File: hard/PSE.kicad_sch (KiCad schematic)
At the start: 0 parts

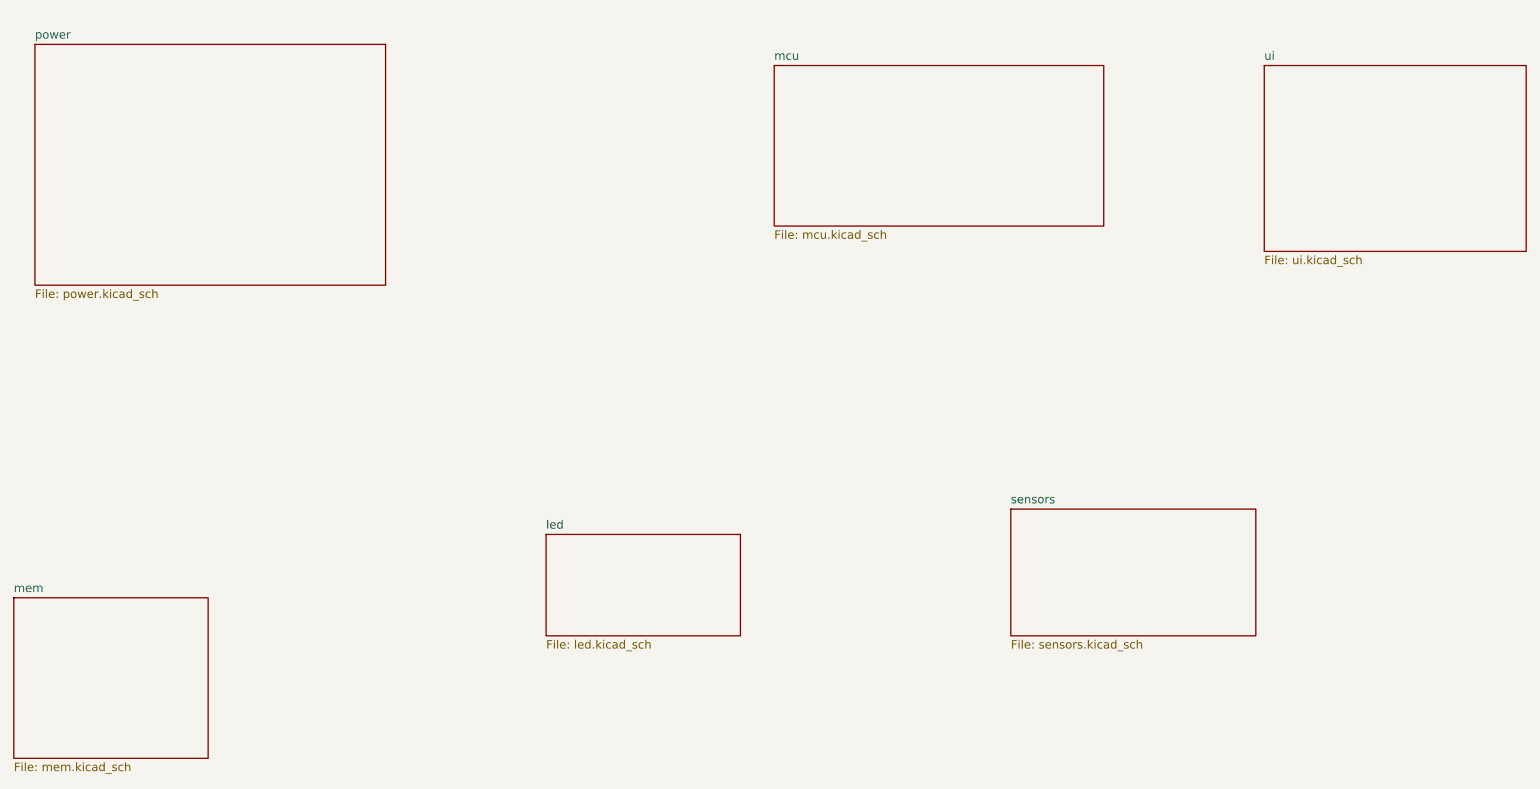
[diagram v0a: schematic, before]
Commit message: update
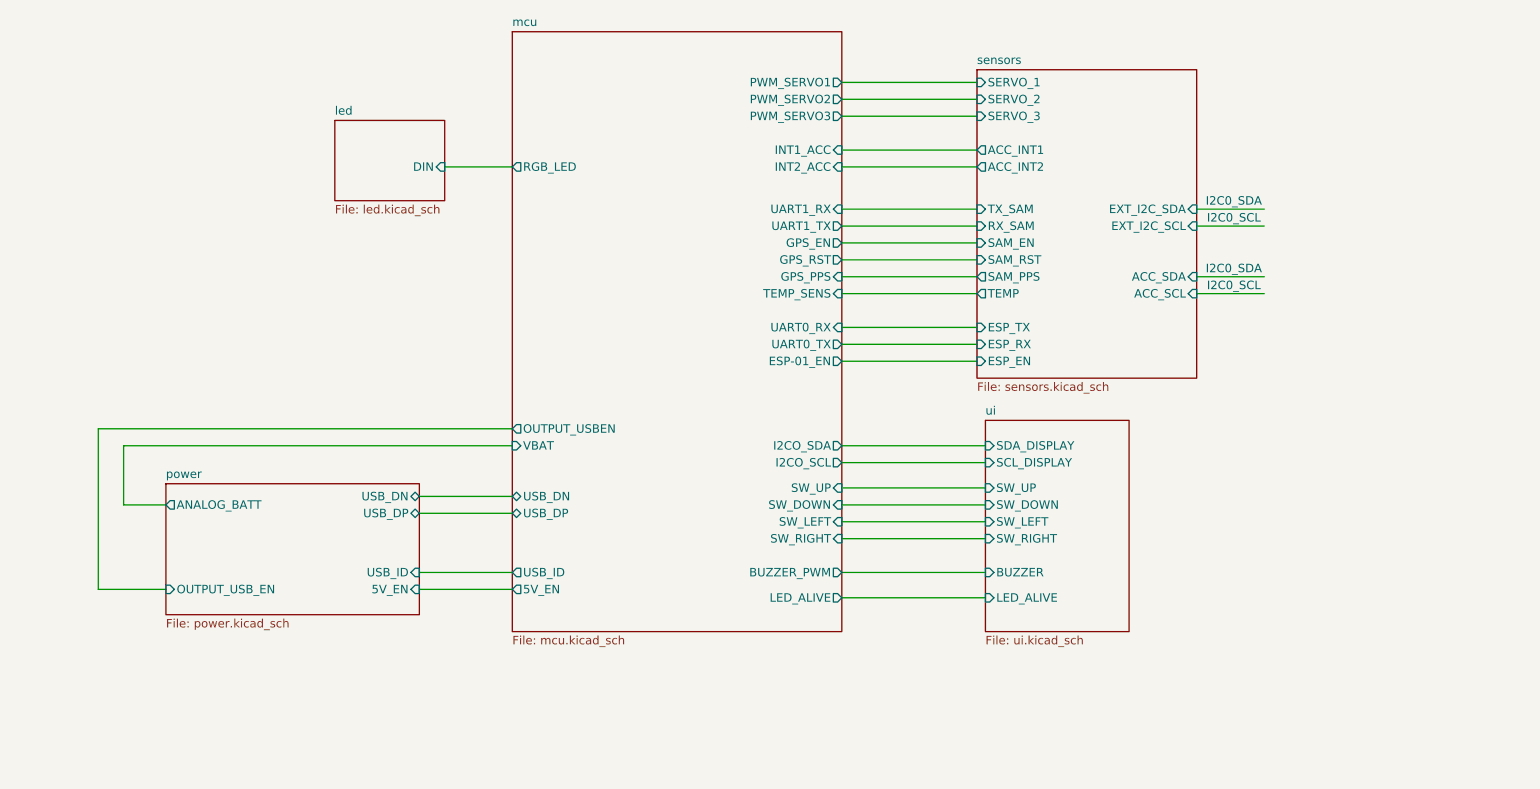
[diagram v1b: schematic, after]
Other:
- removed sheet mem
- sheet led ports: added DIN; removed none
- sheet mcu ports: added 5V_EN, BUZZER_PWM, ESP-01_EN, GPS_EN, GPS_PPS, GPS_RST, I2CO_SCL, I2CO_SDA, INT1_ACC, INT2_ACC, LED_ALIVE, OUTPUT_USBEN, PWM_SERVO1, PWM_SERVO2, PWM_SERVO3, RGB_LED, SW_DOWN, SW_LEFT, SW_RIGHT, SW_UP, TEMP_SENS, UART0_RX, UART0_TX, UART1_RX, UART1_TX, USB_DN, USB_DP, USB_ID, VBAT; removed none
- sheet power ports: added 5V_EN, ANALOG_BATT, OUTPUT_USB_EN, USB_DN, USB_DP, USB_ID; removed none
- sheet sensors ports: added ACC_INT1, ACC_INT2, ACC_SCL, ACC_SDA, ESP_EN, ESP_RX, ESP_TX, EXT_I2C_SCL, EXT_I2C_SDA, RX_SAM, SAM_EN, SAM_PPS, SAM_RST, SERVO_1, SERVO_2, SERVO_3, TEMP, TX_SAM; removed none
- sheet ui ports: added BUZZER, LED_ALIVE, SCL_DISPLAY, SDA_DISPLAY, SW_DOWN, SW_LEFT, SW_RIGHT, SW_UP; removed none
- note added: "I2C0_SCL"
- note added: "I2C0_SDA"
